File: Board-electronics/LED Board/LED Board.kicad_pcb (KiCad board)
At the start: 2 copper layers, 153.4 x 43.1 mm, 49 parts, among them J1 CONN_02X06, M2.5 MountingHole_2.7mm_M2.5_Pad, Q1 PN2222A, Q2 PN2222A, Q3 PN2222A

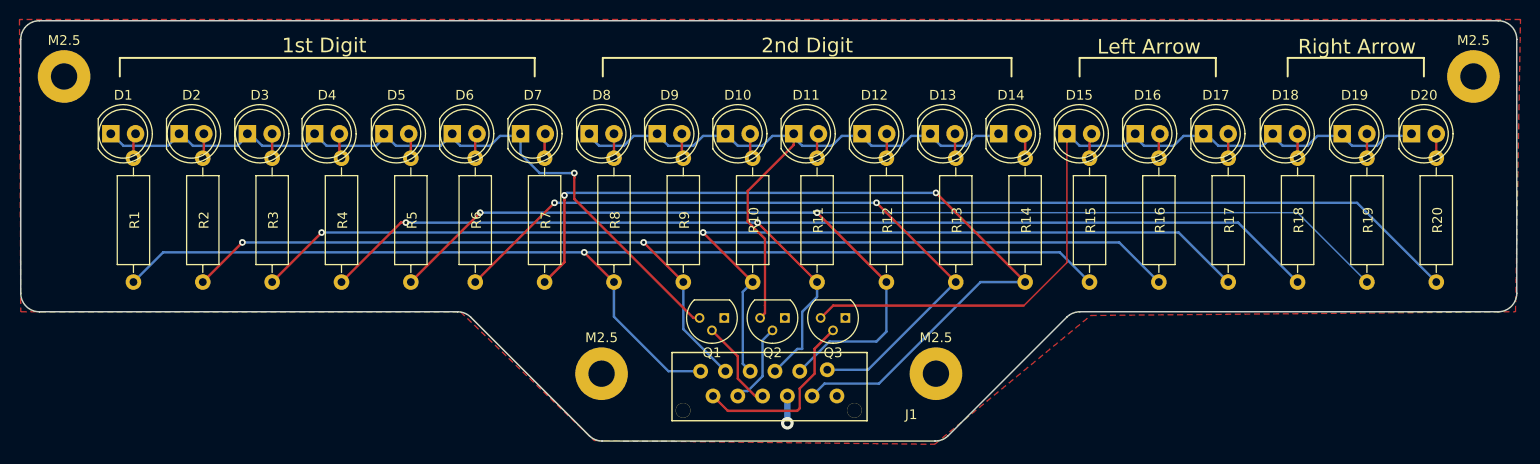
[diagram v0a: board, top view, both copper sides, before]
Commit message: more tweaking for perfection
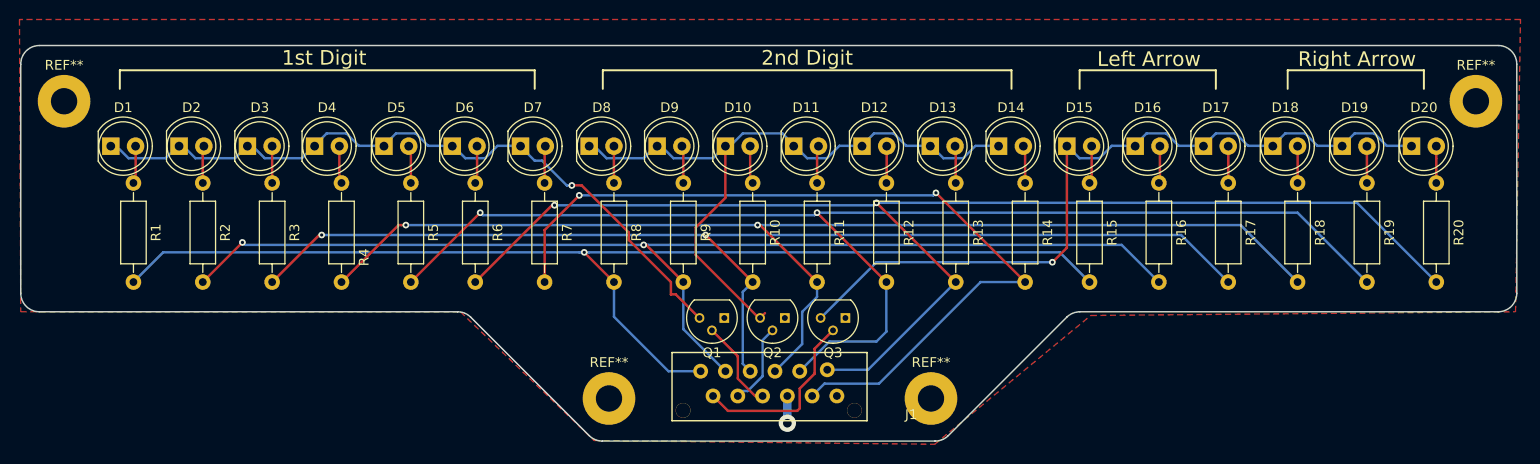
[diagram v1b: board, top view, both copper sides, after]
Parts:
- removed M2.5 (x4): MountingHole_2.7mm_M2.5_Pad, Mounting_Holes:MountingHole_2.7mm_M2.5_Pad
- removed REF***: ESD-Logo_13.2x12mm_SilkScreen, Symbols:ESD-Logo_13.2x12mm_SilkScreen
- added REF**: MountingHole_2.7mm_M2.5_Pad, Mounting_Holes:MountingHole_2.7mm_M2.5_Pad, F.Cu at (238.8, 115.6)
- added REF**: MountingHole_2.7mm_M2.5_Pad, Mounting_Holes:MountingHole_2.7mm_M2.5_Pad, F.Cu at (205.7, 115.6)
- added REF**: MountingHole_2.7mm_M2.5_Pad, Mounting_Holes:MountingHole_2.7mm_M2.5_Pad, F.Cu at (149.9, 85.1)
- added REF**: MountingHole_2.7mm_M2.5_Pad, Mounting_Holes:MountingHole_2.7mm_M2.5_Pad, F.Cu at (294.6, 85.1)
- R1, R10, R11, R12, R13, R14, R15, R16, R17, R18, R19, R2, R20, R3, R4, R5, R6, R7, R8, R9: footprint Resistors_THT:R_Axial_DIN0309_L9.0mm_D3.2mm_P12.70mm_Horizontal -> Resistors_THT:R_Axial_DIN0207_L6.3mm_D2.5mm_P10.16mm_Horizontal
- moved R1 2.54 mm to (157.0, 93.5)
- moved R10 2.54 mm to (220.5, 93.5)
- moved R11 2.54 mm to (227.1, 93.5)
- moved R12 2.54 mm to (234.2, 93.5)
- moved R13 2.54 mm to (241.3, 93.5)
- moved R14 2.54 mm to (248.4, 93.5)
- moved R15 2.54 mm to (255.0, 93.5)
- moved R16 2.54 mm to (262.1, 93.5)
- moved R17 2.54 mm to (269.2, 93.5)
- moved R18 2.54 mm to (276.4, 93.5)
- moved R19 2.54 mm to (283.5, 93.5)
- moved R2 2.54 mm to (164.1, 93.5)
- moved R20 2.54 mm to (290.6, 93.5)
- moved R3 2.54 mm to (171.2, 93.5)
- moved R4 2.54 mm to (178.3, 93.5)
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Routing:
- net Net-(D15-Pad1): track 82.5 -> 80.1 mm, vias 0 -> 1
- net Net-(D1-Pad1): track 78.5 -> 76.4 mm
- net Net-(D4-Pad2): track 2.84 -> 4.28 mm
- net Net-(D1-Pad2): track 2.91 -> 4.28 mm
- net Net-(D10-Pad2): track 2.61 -> 3.88 mm
- net Net-(D20-Pad2): track 2.51 -> 3.78 mm
- net Net-(D19-Pad2): track 2.51 -> 3.78 mm
- net Net-(D18-Pad2): track 2.51 -> 3.78 mm
- net Net-(D17-Pad2): track 2.51 -> 3.78 mm
- net Net-(D2-Pad2): track 2.80 -> 3.94 mm
- net Net-(D3-Pad2): track 2.73 -> 3.81 mm
- net Net-(D11-Pad2): track 2.77 -> 3.84 mm
- net Net-(D8-Pad2): track 2.73 -> 3.78 mm
- net Net-(D12-Pad2): track 2.74 -> 3.79 mm
- net Net-(D13-Pad2): track 2.77 -> 3.81 mm
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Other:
- board size 153.4 x 43.1 mm -> 153.4 x 40.6 mm
- net class Default: trace_width 0.1524 -> 0.254
- rule trace_min: 0.1524 -> 0.254
